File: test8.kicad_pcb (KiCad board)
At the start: 2 copper layers, 28.5 x 23.5 mm, 4 parts, among them J1 Conn_01x02_Pin, U1 74HC165, U2 74HC165, U3 ESP32-WROOM-32

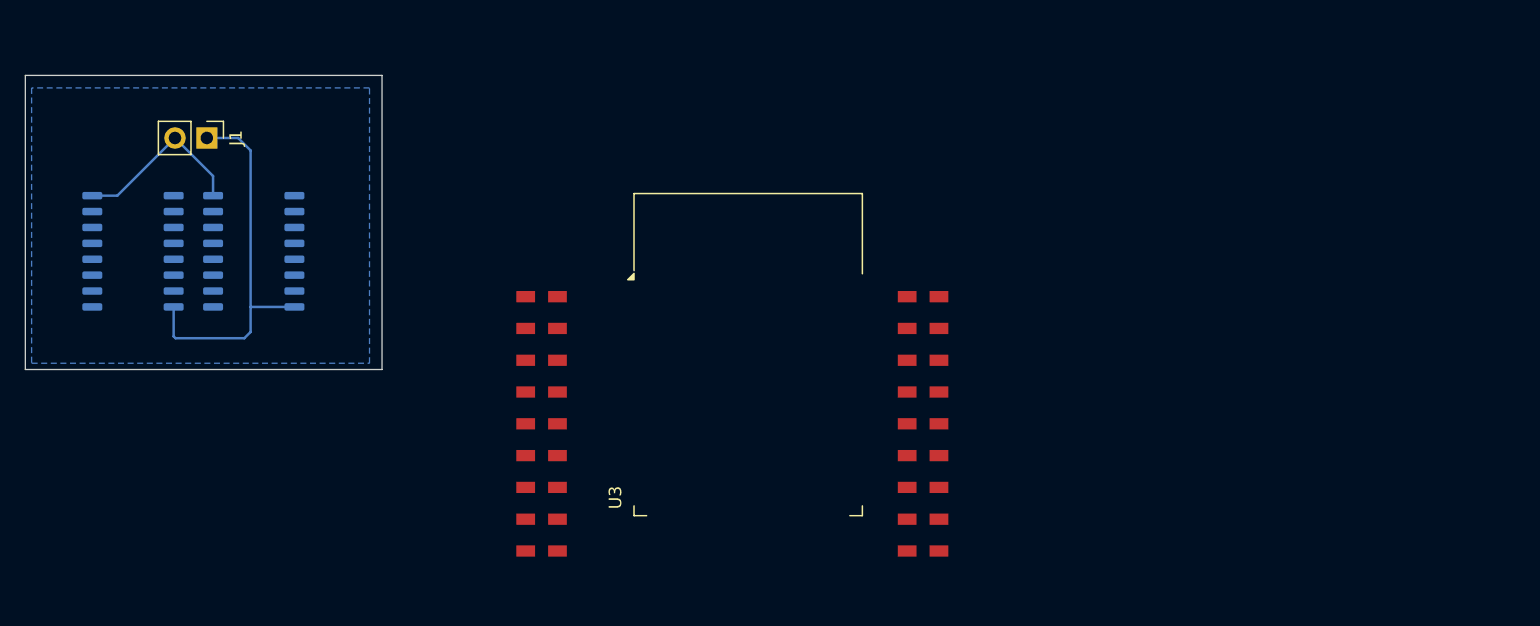
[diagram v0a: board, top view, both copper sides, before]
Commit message: process
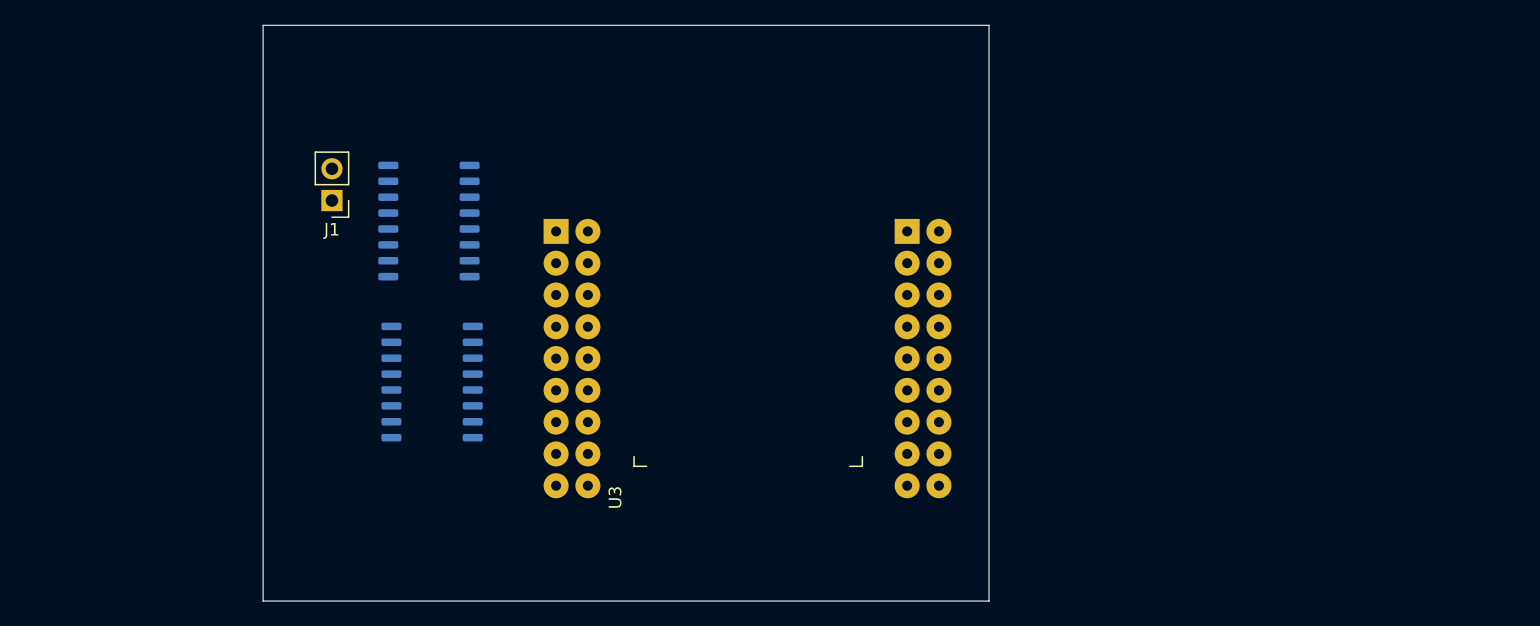
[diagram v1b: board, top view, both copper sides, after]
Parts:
- moved U1 26.1 mm to (120.5, 108.0)
- moved U2 14.2 mm to (120.2, 95.1)
- moved J1 11.2 mm to (112.5, 93.5), turned to 180 degrees
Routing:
- net GND: track 30.7 -> 0.00 mm
- net +3.3V: track 14.4 -> 0.00 mm
- removed copper zone on B.Cu, net GND
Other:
- board size 28.5 x 23.5 mm -> 58 x 46 mm

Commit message: xz
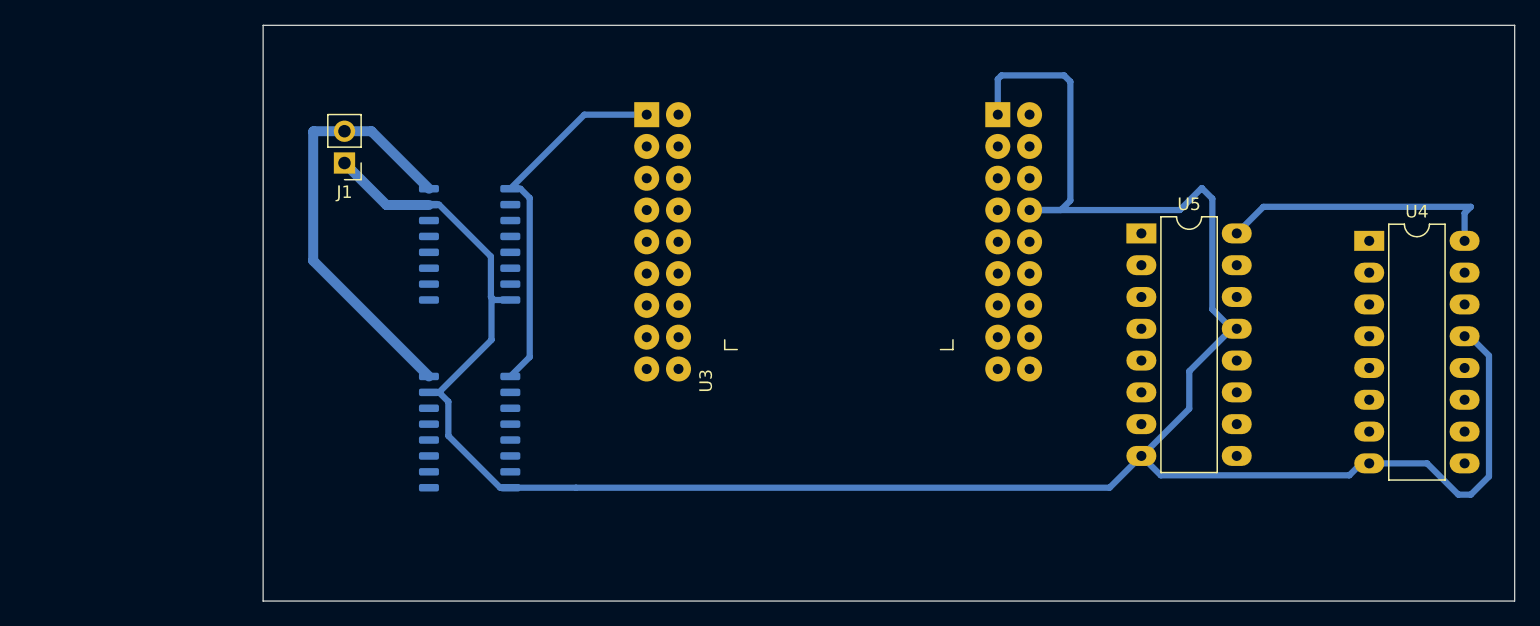
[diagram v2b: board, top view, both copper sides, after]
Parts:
- added U4: 74HC595, Package_DIP:DIP-16_W7.62mm_LongPads, F.Cu at (195.4, 96.7)
- added U5: 74HC595, Package_DIP:DIP-16_W7.62mm_LongPads, F.Cu at (177.2, 96.1)
- moved U2 17.2 mm to (123.5, 112.0)
- moved U3 11.8 mm to (153.0, 99.5)
- moved U1 11.4 mm to (123.5, 97.0)
- moved J1 3.16 mm to (113.5, 90.5)
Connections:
- U1 pad 1: unconnected-(U1-~{PL}-Pad1) -> CS_165
- U1 pad 10: unconnected-(U1-DS-Pad10) -> Net-(U1-DS)
- U1 pad 15: unconnected-(U1-~{CE}-Pad15) -> GND
- U1 pad 2: unconnected-(U1-CP-Pad2) -> CLK_165
- U1 pad 9: unconnected-(U1-Q7-Pad9) -> MISO_165
- U2 pad 1: unconnected-(U2-~{PL}-Pad1) -> CS_165
- U2 pad 15: unconnected-(U2-~{CE}-Pad15) -> GND
- U2 pad 2: unconnected-(U2-CP-Pad2) -> CLK_165
- U2 pad 9: unconnected-(U2-Q7-Pad9) -> Net-(U1-DS)
- U3 pad 13: unconnected-(U3-IO14-Pad13) -> Net-(U3-IO14)
- U3 pad 16: unconnected-(U3-IO13-Pad16) -> Net-(U3-IO13)
- U3 pad 23: unconnected-(U3-IO15-Pad23) -> Net-(U3-IO15)
- U3 pad 30: unconnected-(U3-IO18-Pad30) -> CLK_165
- U3 pad 31: unconnected-(U3-IO19-Pad31) -> MISO_165
- U3 pad 5: unconnected-(U3-SENSOR_VN-Pad5) -> CS_165
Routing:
- net GND: track 0.00 -> 196.8 mm
- net +3.3V: track 0.00 -> 34.6 mm
- net CS_165: track 0.00 -> 30.1 mm
- net +5V: track 0.00 -> 22.5 mm
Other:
- board size 58 x 46 mm -> 100 x 46 mm
